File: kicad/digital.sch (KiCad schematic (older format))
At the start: 8 parts

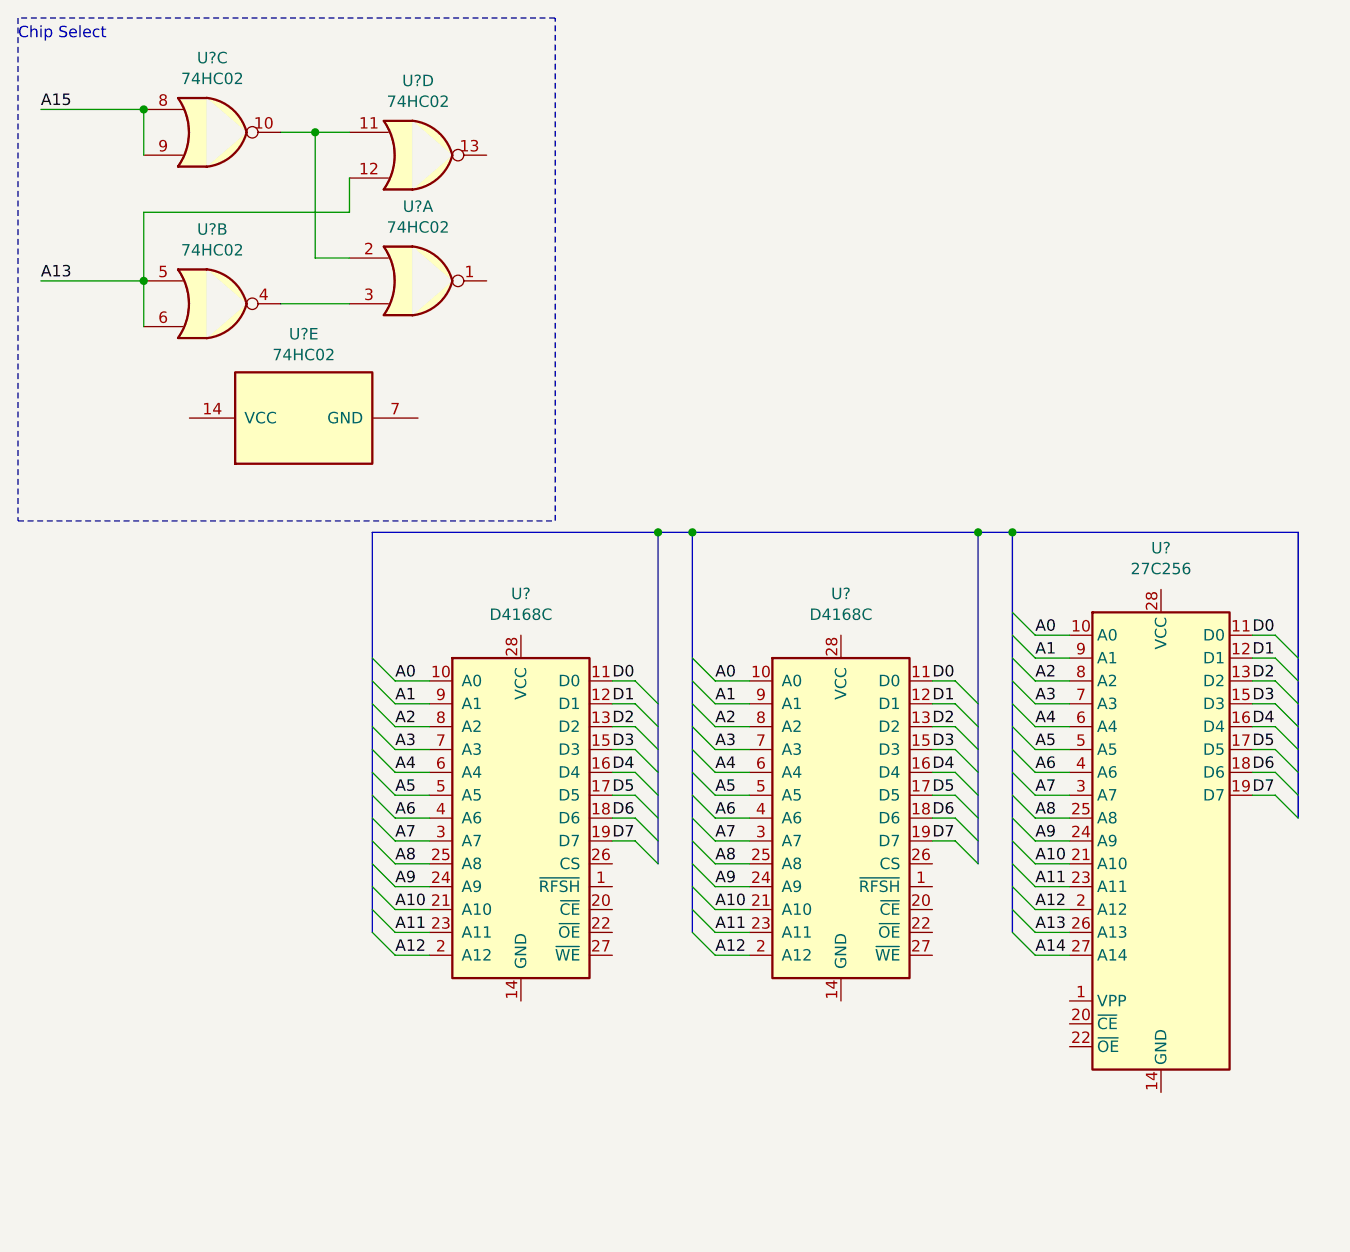
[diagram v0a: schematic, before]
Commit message: a
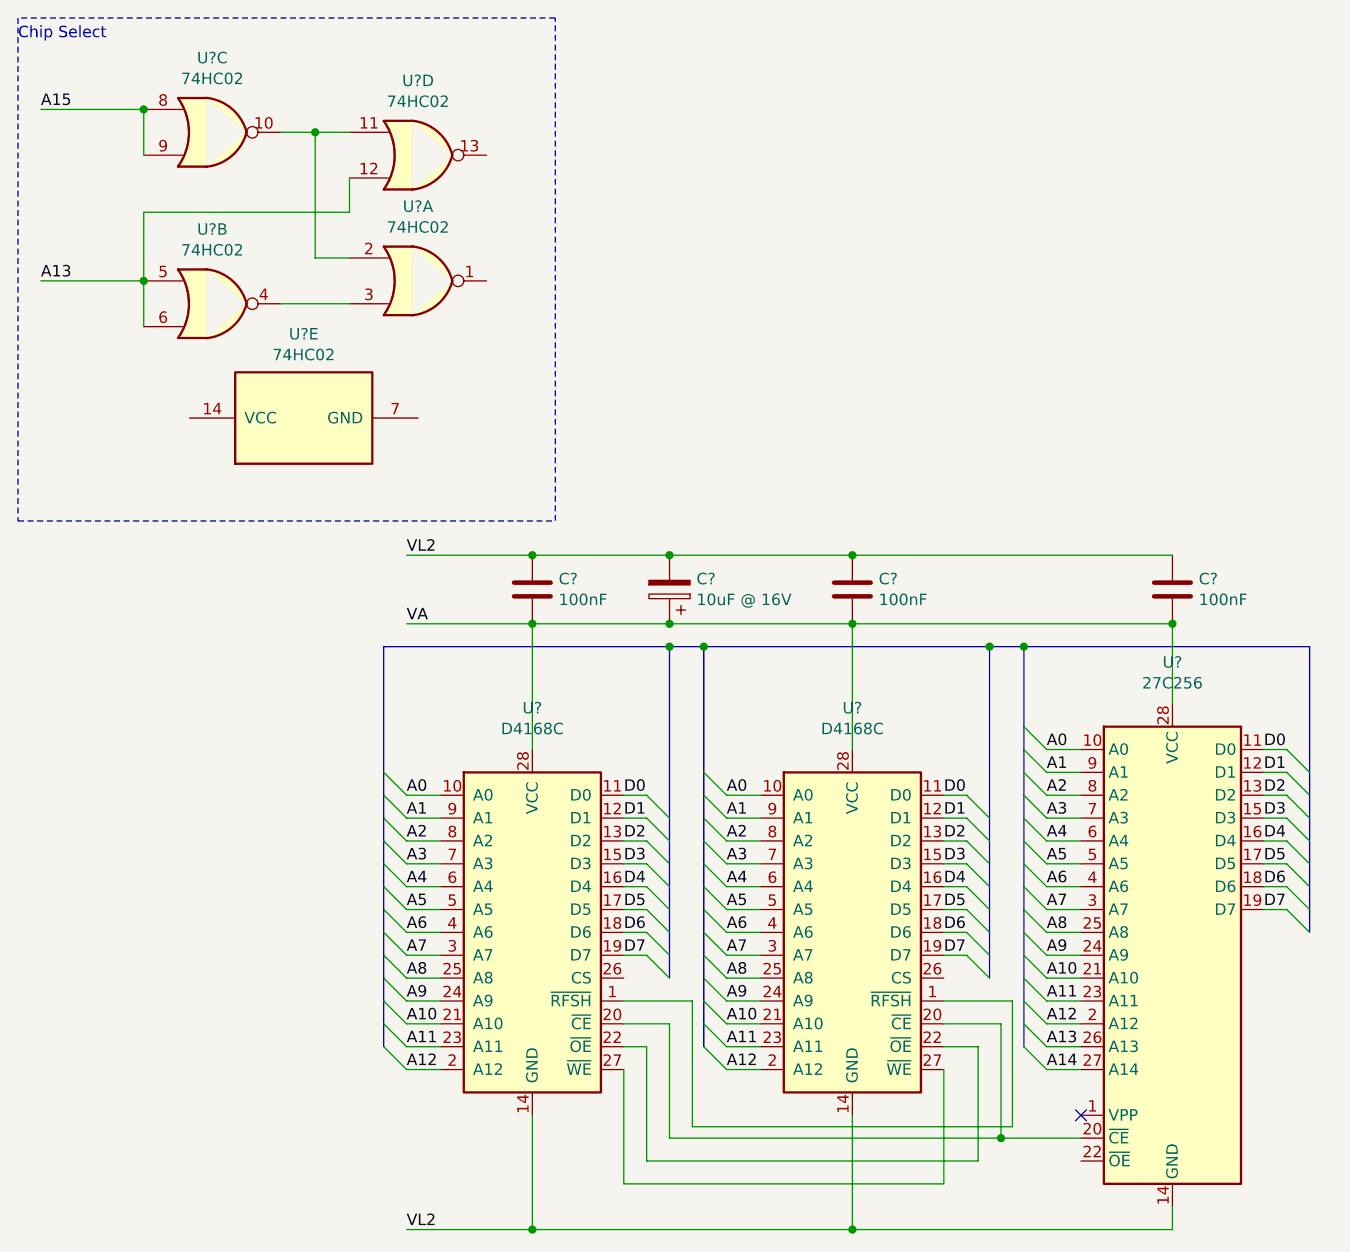
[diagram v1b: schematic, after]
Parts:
- added C? (x3): 100nF, symbol Device:C
- added C?: 10uF @ 16V, symbol Device:CP
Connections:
- net VL2: now reaches U?.14 (GND)
- net VL2: now also U?.14 (GND), U?.14 (GND), C?.1, C?.1, C?.1, C?.2
- net at U?.20 (~CE): now also U?.20 (~CE), U?.20 (~CE)
- net VA: now reaches U?.28 (VCC)
- net VA: now also U?.28 (VCC), U?.28 (VCC), C?.1, C?.2, C?.2, C?.2
- net at U?.1 (~RFSH): now also U?.1 (~RFSH)
- net at U?.22 (~OE): now also U?.22 (~OE)
- net at U?.27 (~WE): now also U?.27 (~WE)
- no-connect marks 0 -> 1
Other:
- moved on the sheet: U?

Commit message: cleanup
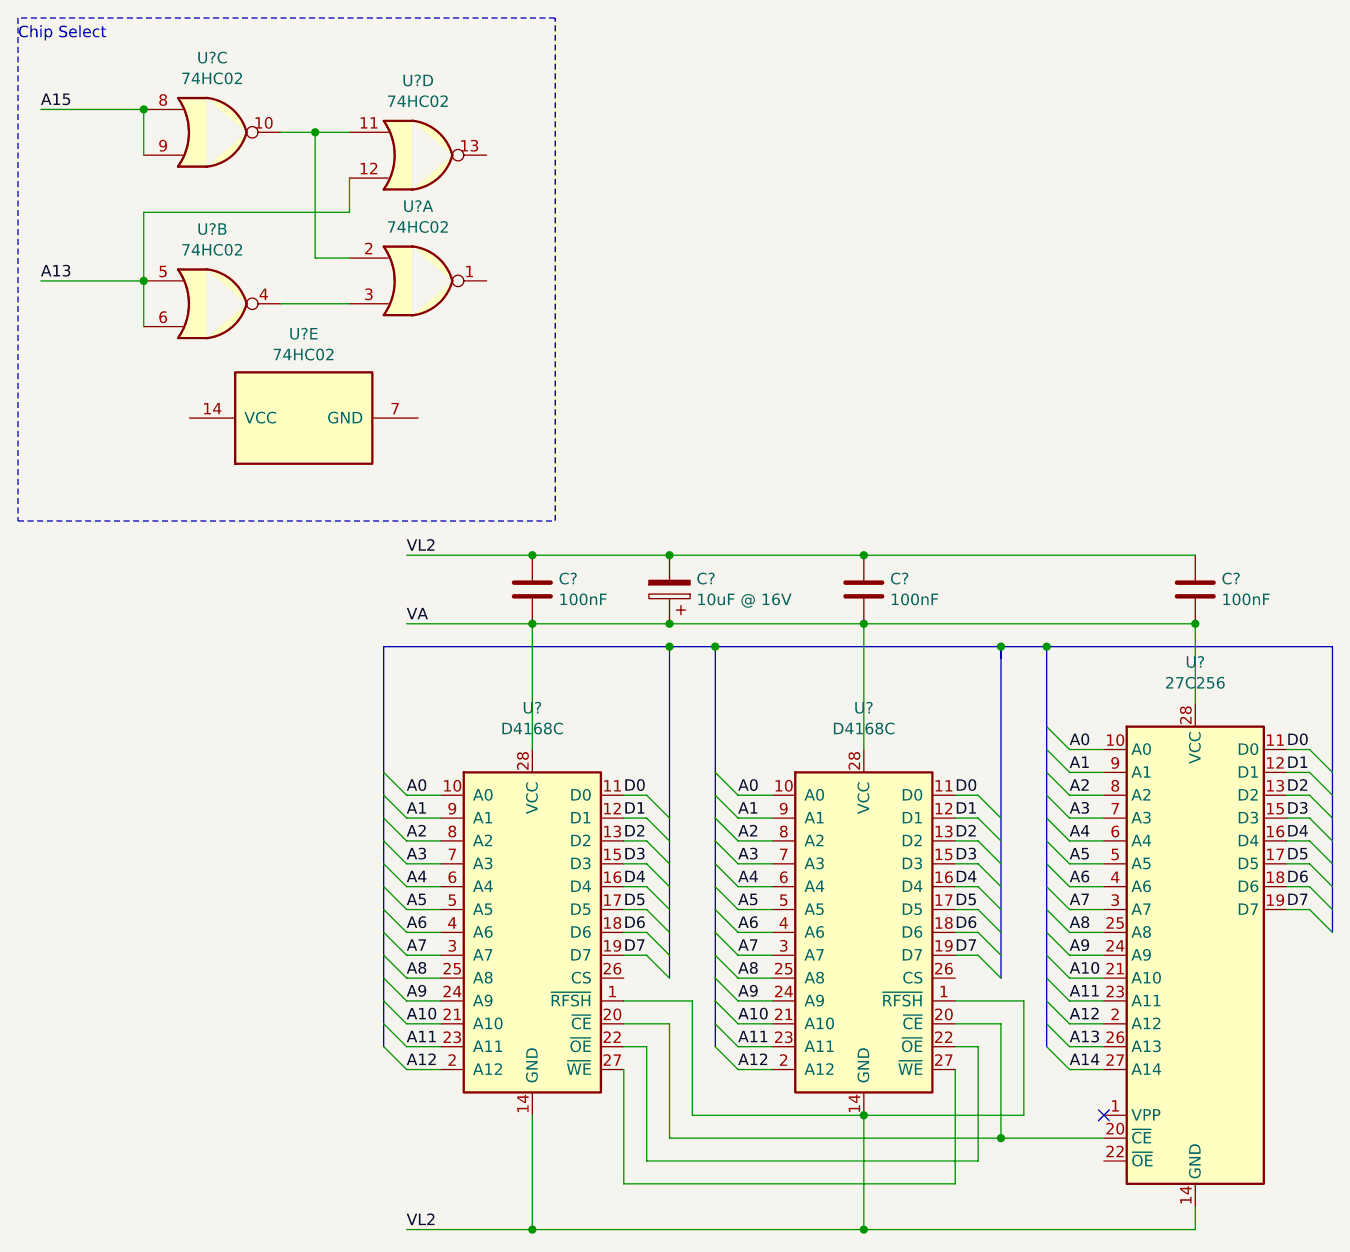
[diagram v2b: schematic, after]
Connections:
- net VL2: now also U?.1 (~RFSH), U?.1 (~RFSH)
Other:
- moved on the sheet: C?, U?
